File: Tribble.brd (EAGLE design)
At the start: 154.5 x 47.2 mm, 121 parts, among them J1 10118193-0001LF, J2 68602-406HLF, J3 SJ1-2503A, J4 RJHSE-5381, J5 SJ1-2503A, J6 SJ1-2503A, J7 HFW6R-2STE1LF, P1 TC33X-2, U1 AT90USB1287-MU, U10 IP4234CZ6, U11 AT90USB1287-AU, U12 FDS6679AZ, U13 MCP9701T-E/TT, U14 MCP9701T-E/TT, U15 BC847BMTF, U16 FDV304P, U2 MMDT3904, U3 BTM7755, U4 MC78M05CDTG, U6 ISL8483, U8 LMP8640MK-F/NOPB, U9 MCP9701T-E/TT, X1 TSX-3225 16.0000MF10U-B0

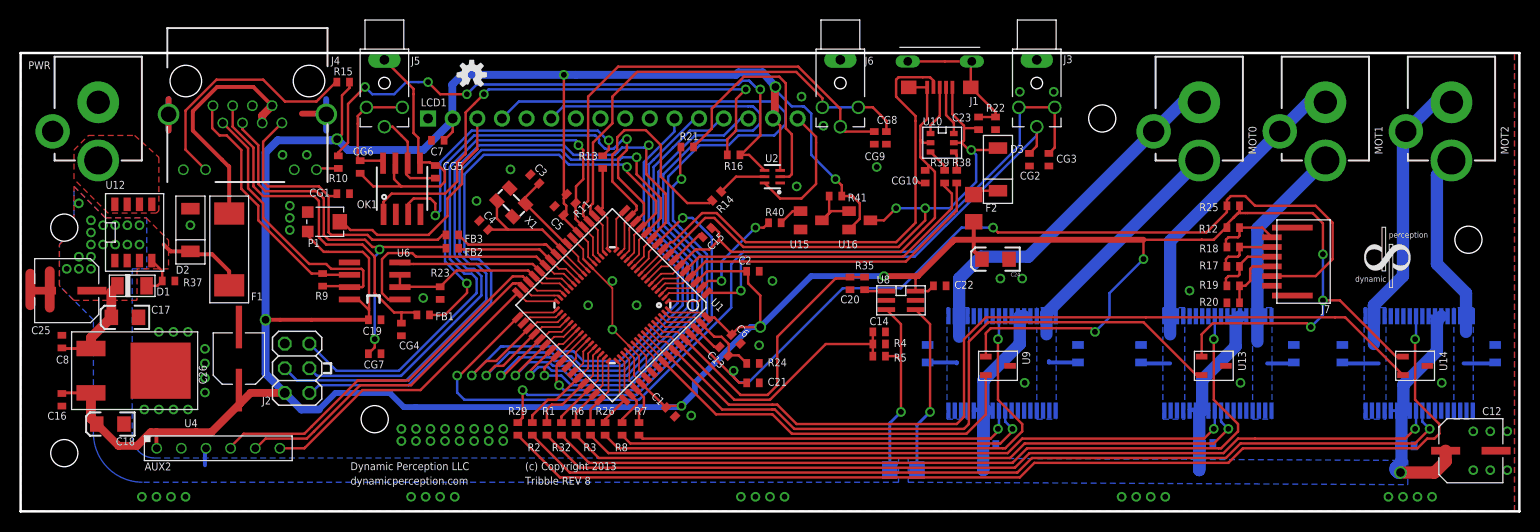
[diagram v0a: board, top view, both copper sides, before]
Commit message: tagged loads of PCBs and made sure BOMs where up to date
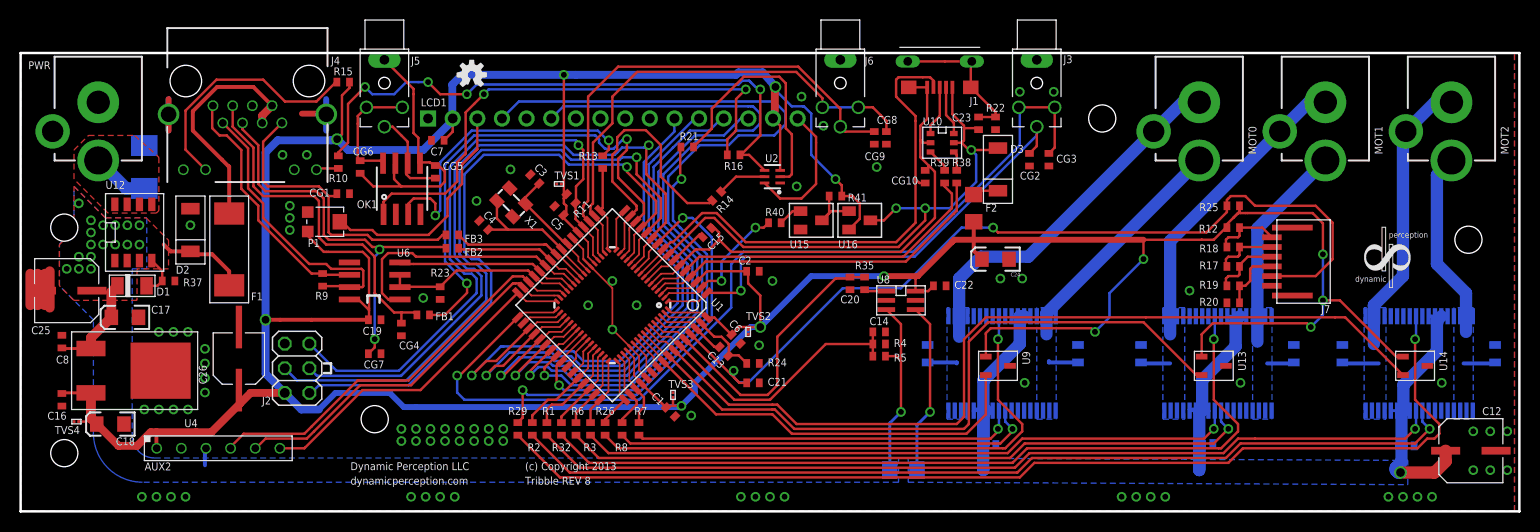
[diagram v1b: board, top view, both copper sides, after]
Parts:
- added D4: P6SMB30CAT3G, PP_Passives:DO-214AA
- added TVS1, TVS2, TVS3, TVS4: ESD11B5.0ST5G, PP_Passives:DSN-2
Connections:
- net +5V: now also TVS1.P$2, TVS2.P$2, TVS3.P$2, TVS4.P$2
- net GND: now also D4.A, TVS1.P$1, TVS2.P$1, TVS3.P$1, TVS4.P$1
- net VIN_J: now also D4.C
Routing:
- net GND: track 37.6 -> 44.1 mm
- net VIN_J: track 0.00 -> 5.94 mm
- net +5V: track 438.0 -> 441.1 mm
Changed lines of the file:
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@@
 <element name="C5" library="parkers_parts" package="0402_CAP" value=".1uF" x="-18.5" y="2.75" rot="R135"/>
 <element name="C6" library="parkers_parts" package="0402_CAP" value=".1uF" x="-0.25" y="-10.5" smashed="yes" rot="R315">
-<attribute name="NAME" x="-0.308965625" y="-9.453203125" size="0.8128" layer="25" font="vector" rot="R315"/>
+<attribute name="NAME" x="-1.058965625" y="-8.953203125" size="0.8128" layer="25" font="vector" rot="R315"/>
 </element>
 <element name="R5" library="parkers_parts" package="0402_RES" value="20K" x="14.5" y="-12.25" smashed="yes">
@@
 </element>
 <element name="C26" library="PP_Passives" package="5MM_CAP_SMD" value="100uF" x="-51.5" y="-12.5" rot="R90"/>
+<element name="TVS1" library="PP_Passives" package="DSN-2" value="ESD11B5.0ST5G" x="-18.5" y="5.5"/>
+<element name="TVS2" library="PP_Passives" package="DSN-2" value="ESD11B5.0ST5G" x="1" y="-9.75" smashed="yes" rot="R90">
+<attribute name="NAME" x="0.78" y="-8.53" size="0.8128" layer="21" font="vector"/>
+</element>
+<element name="TVS3" library="PP_Passives" package="DSN-2" value="ESD11B5.0ST5G" x="-6.75" y="-16.25" smashed="yes" rot="R270">
+<attribute name="NAME" x="-7.22" y="-15.53" size="0.8128" layer="21" font="vector"/>
+</element>
+<element name="TVS4" library="PP_Passives" package="DSN-2" value="ESD11B5.0ST5G" x="-68.25" y="-19" smashed="yes">
+<attribute name="NAME" x="-70.47" y="-20.28" size="0.8128" layer="21" font="vector"/>
+</element>
+<element name="D4" library="PP_Passives" package="DO-214AA" value="P6SMB30CAT3G" x="-61.25" y="7.25" rot="MR90"/>
 </elements>
 <signals>
@@
 <via x="3.81" y="15.5" extent="1-16" drill="0.8"/>
 <wire x1="-0.70961875" y1="-10.040378125" x2="0.080759375" y2="-9.25" width="0.254" layer="1"/>
-<wire x1="0.080759375" y1="-9.25" x2="2.25" y2="-9.25" width="0.254" layer="1"/>
+<wire x1="0.080759375" y1="-9.25" x2="1.25" y2="-9.25" width="0.254" layer="1"/>
 <via x="2.25" y="-9.25" extent="1-16" drill="0.8"/>
+<wire x1="1.25" y1="-9.25" x2="2.25" y2="-9.25" width="0.254" layer="1"/>
 <wire x1="2.25" y1="-9.25" x2="1.25" y2="-9.25" width="0.6096" layer="16"/>
 <wire x1="1.25" y1="-9.25" x2="-4.5" y2="-15" width="0.6096" layer="16"/>
@@
 <wire x1="-0.25" y1="16.75" x2="0" y2="17" width="0.8128" layer="16"/>
 <wire x1="0" y1="17" x2="2.5" y2="17" width="0.8128" layer="16"/>
-<wire x1="-7.45961875" y1="-17.381546875" x2="-5.881546875" y2="-17.381546875" width="0.254" layer="1"/>
+<wire x1="-7.45961875" y1="-17.381546875" x2="-6.75" y2="-17.381546875" width="0.254" layer="1"/>
+<wire x1="-6.75" y1="-17.381546875" x2="-5.881546875" y2="-17.381546875" width="0.254" layer="1"/>
 <wire x1="-5.881546875" y1="-17.381546875" x2="-5.875" y2="-17.375" width="0.254" layer="1"/>
 <via x="-5.875" y="-17.375" extent="1-16" drill="0.6"/>
@@
 <wire x1="4.3" y1="6.9" x2="4.3" y2="11.51" width="0.254" layer="1"/>
 <wire x1="4.3" y1="11.51" x2="3.56" y2="12.25" width="0.254" layer="1"/>
-<wire x1="-18" y1="4" x2="-18" y2="16.75" width="0.254" layer="1"/>
+<wire x1="-18" y1="4" x2="-18" y2="5.5" width="0.254" layer="1"/>
 <via x="-18" y="16.75" extent="1-16" drill="0.6"/>
+<wire x1="-18" y1="5.5" x2="-18" y2="16.75" width="0.254" layer="1"/>
 <wire x1="-18" y1="16.75" x2="-16.75" y2="16.75" width="0.254" layer="16"/>
 <contactref element="R15" pad="1"/>
@@
 <wire x1="60.250003125" y1="1.439340625" x2="60.250003125" y2="-1.75" width="0.254" layer="1"/>
 <wire x1="51.650003125" y1="2.65" x2="51.650003125" y2="3.25" width="0.254" layer="1"/>
-<wire x1="-66.750003125" y1="-16.035" x2="-66.750003125" y2="-18.65" width="1.016" layer="1"/>
+<wire x1="-66.750003125" y1="-16.035" x2="-66.750003125" y2="-18.5" width="1.016" layer="1"/>
+<wire x1="-66.750003125" y1="-18.5" x2="-66.750003125" y2="-18.65" width="1.016" layer="1"/>
 <wire x1="-66.750003125" y1="-18.65" x2="-66.150003125" y2="-19.25" width="1.016" layer="1"/>
 <wire x1="-38.15" y1="-8.5" x2="-44" y2="-8.5" width="0.4064" layer="1"/>
@@
 <wire x1="-51.5" y1="-15.75" x2="-51.5" y2="-16.999996875" width="0.6096" layer="1"/>
 <wire x1="-51.5" y1="-16.999996875" x2="-51.375" y2="-17.124996875" width="0.6096" layer="1"/>
+<contactref element="TVS4" pad="P$2"/>
+<contactref element="TVS1" pad="P$2"/>
+<contactref element="TVS2" pad="P$2"/>
+<contactref element="TVS3" pad="P$2"/>
+<wire x1="-18.265" y1="5.5" x2="-18" y2="5.5" width="0.254" layer="1"/>
+<wire x1="1" y1="-9.515" x2="1" y2="-9.25" width="0.254" layer="1"/>
+<wire x1="1" y1="-9.25" x2="1.25" y2="-9.25" width="0.254" layer="1"/>
+<wire x1="-6.75" y1="-16.485" x2="-6.75" y2="-17.381546875" width="0.254" layer="1"/>
+<wire x1="-68.015" y1="-19" x2="-67.250003125" y2="-19" width="0.254" layer="1"/>
+<wire x1="-67.250003125" y1="-19" x2="-66.750003125" y2="-18.5" width="0.254" layer="1"/>
 </signal>
 <signal name="GND">
@@
 <wire x1="-71" y1="-3.5" x2="-71" y2="-7.25" width="1.016" layer="1"/>
 <contactref element="C25" pad="NEG"/>
+<wire x1="-72.25" y1="-3.75" x2="-72.25" y2="-7" width="1.016" layer="1"/>
+<wire x1="-71.5" y1="-3.75" x2="-71.5" y2="-7" width="1.016" layer="1"/>
+<contactref element="TVS4" pad="P$1"/>
+<contactref element="TVS3" pad="P$1"/>
+<contactref element="TVS2" pad="P$1"/>
+<contactref element="TVS1" pad="P$1"/>
+<contactref element="D4" pad="A"/>
 </signal>
 <signal name="AREF" class="4">
@@
 <vertex x="-59.750003125" y="2.75"/>
 </polygon>
+<contactref element="D4" pad="C"/>
+<wire x1="-61.25" y1="5.04" x2="-63.12" y2="5.04" width="1.27" layer="16"/>
+<wire x1="-63.12" y1="5.04" x2="-66" y2="7.92" width="1.27" layer="16"/>
 </signal>
 <signal name="N$3">

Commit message: Revert to REV 7 of Tribble
Did not need the board fixes in REV 8 of the pcb.
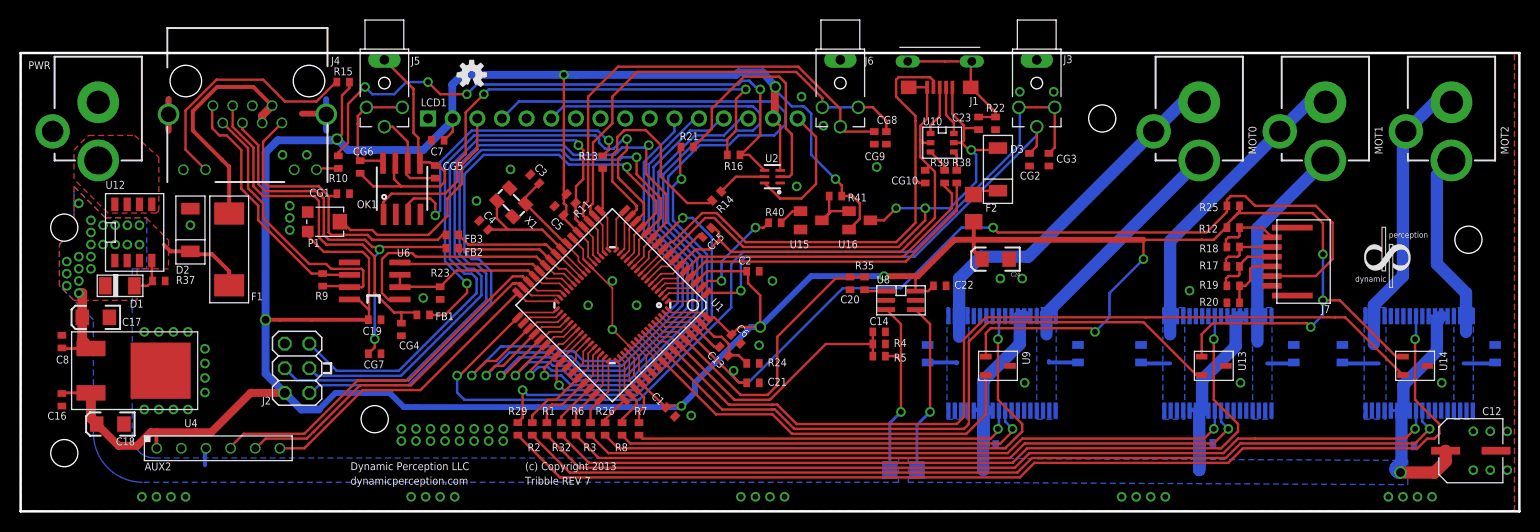
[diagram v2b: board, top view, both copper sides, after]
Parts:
- removed C25: 100uF, PP_Passives:6.3MM_CAP_SMD
- removed C26: 100uF, PP_Passives:5MM_CAP_SMD
- removed D4: P6SMB30CAT3G, PP_Passives:DO-214AA
- removed TVS1, TVS2, TVS3, TVS4: ESD11B5.0ST5G, PP_Passives:DSN-2
- FB1, FB2, FB3: value HZ0402B102R-10 -> LI0402C470R-10
- moved C17 3.00 mm to (-66.3, -8.25)
- moved D1 1.25 mm to (-64.0, -5.00)
- moved R37 1.00 mm to (-59.8, -4.50)
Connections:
- net +5V: no longer C26.P, TVS1.P$2, TVS2.P$2, TVS3.P$2, TVS4.P$2
- net GND: no longer C25.NEG, C26.N, D4.A, TVS1.P$1, TVS2.P$1, TVS3.P$1, TVS4.P$1
- net VIN: no longer C25.POS
- net VIN_J: no longer D4.C
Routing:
- net GND: track 44.1 -> 30.6 mm, vias 81 -> 82
- net VIN_J: track 5.94 -> 0.00 mm
- net +5V: track 441.1 -> 436.6 mm
- net VIN: track 42.1 -> 41.0 mm, vias 18 -> 22
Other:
- board text added: "Tribble REV 7"
- board text removed: "Tribble REV 8"
